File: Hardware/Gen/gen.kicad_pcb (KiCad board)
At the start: 2 copper layers, 153.9 x 62.1 mm, 50 parts, among them J1 Screw_Terminal_01x03, J2 XLR4, J3 XLR3, J4 GAMEN, J5 SHORI, J6 MAE, U1 TPS56339DDCT, U3 TPS560430YDBVR

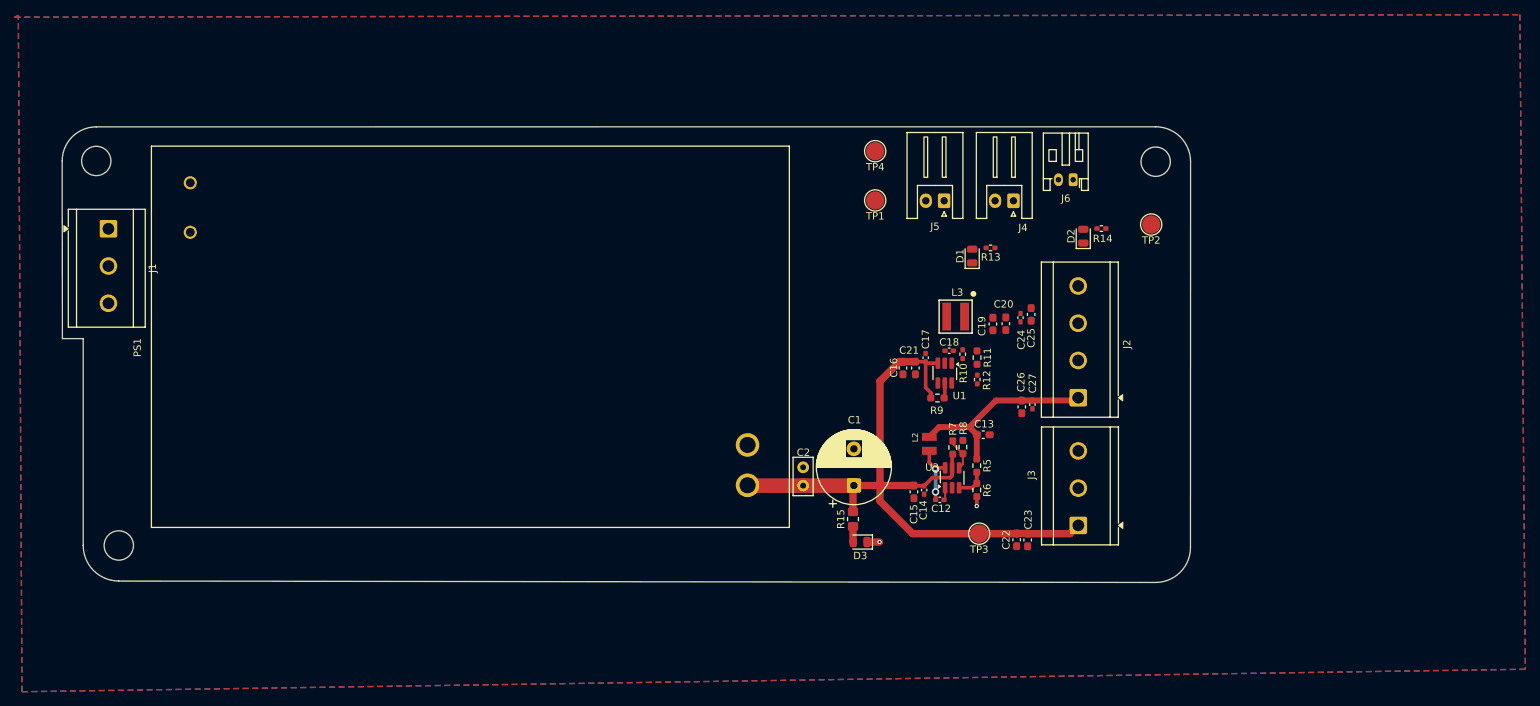
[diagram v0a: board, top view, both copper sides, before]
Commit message: Gen: Layout and routing complete rev 1
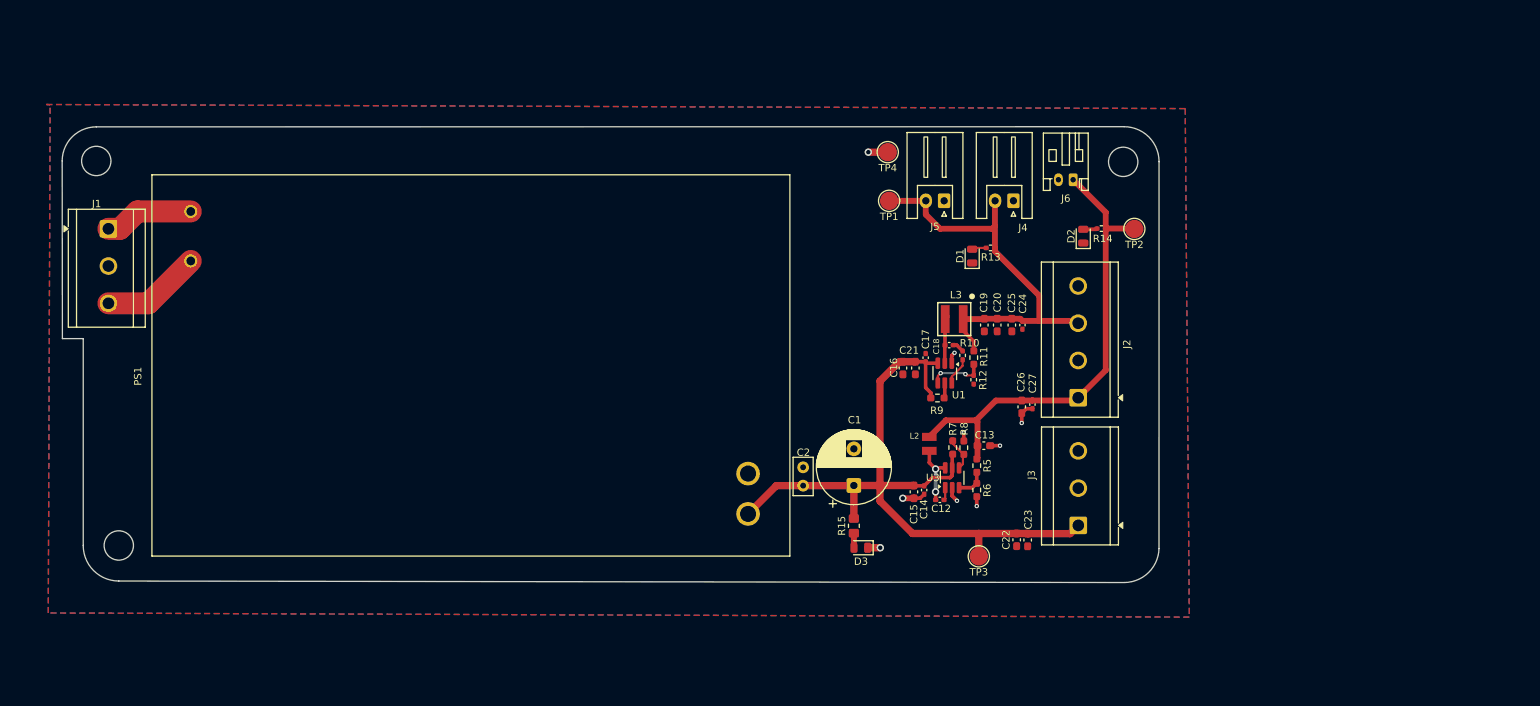
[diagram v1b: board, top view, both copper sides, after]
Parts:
- moved H3 4.43 mm to (214.9, 85.7)
- moved PS1 3.91 mm to (126.0, 113.5)
- moved TP3 3.09 mm to (195.2, 139.5)
- moved C25 3.01 mm to (199.7, 108.0), turned to 90 degrees
- moved TP2 2.38 mm to (216.4, 94.9)
- moved TP1 1.90 mm to (183.0, 91.0)
- moved TP4 1.71 mm to (182.8, 84.4)
- moved C13 1.50 mm to (195.9, 124.4)
- moved C20 1.18 mm to (197.8, 108.0)
- moved C19 1.18 mm to (196.0, 108.0)
- moved C24 1.04 mm to (201.2, 108.0), turned to 90 degrees
- moved R15 0.93 mm to (178.2, 135.4)
- moved D3 0.79 mm to (179.2, 138.4)
- moved C18 0.76 mm to (191.2, 110.7)
- moved R12 0.49 mm to (194.5, 115.5)
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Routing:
- net +5V: track 0.00 -> 57.0 mm
- net +9V: track 27.3 -> 65.0 mm
- net GND: track 2.99 -> 18.0 mm, vias 2 -> 9
- net /ACL: track 0.00 -> 13.6 mm
- net /ACN: track 0.00 -> 12.2 mm
- net Net-(U1-FB): track 0.00 -> 7.69 mm, vias 0 -> 2
- net Net-(U1-SW): track 0.00 -> 6.34 mm
- net /DC_OUT: track 95.4 -> 101.0 mm
- net Net-(U1-BOOT): track 0.00 -> 3.78 mm
- net Net-(D1-A): track 0.00 -> 1.98 mm
- net Net-(D2-A): track 0.00 -> 1.92 mm
- net Net-(C18-Pad2): track 0.00 -> 1.59 mm
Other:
- board size 153.9 x 62.1 mm -> 149.6 x 62.2 mm
